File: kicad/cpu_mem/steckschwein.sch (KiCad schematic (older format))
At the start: 29 parts, among them P1 CONN_02X04, P3 CONN_01X03, P4 CONN_02X02, SW1 SW_PUSH, U1 W65C02SP, U2 LM555N, U3 74HCT00, U4 74LS393, U6 28C256, U7 HM62256BLP-7, U8 HM62256BLP-7, X1 OSC

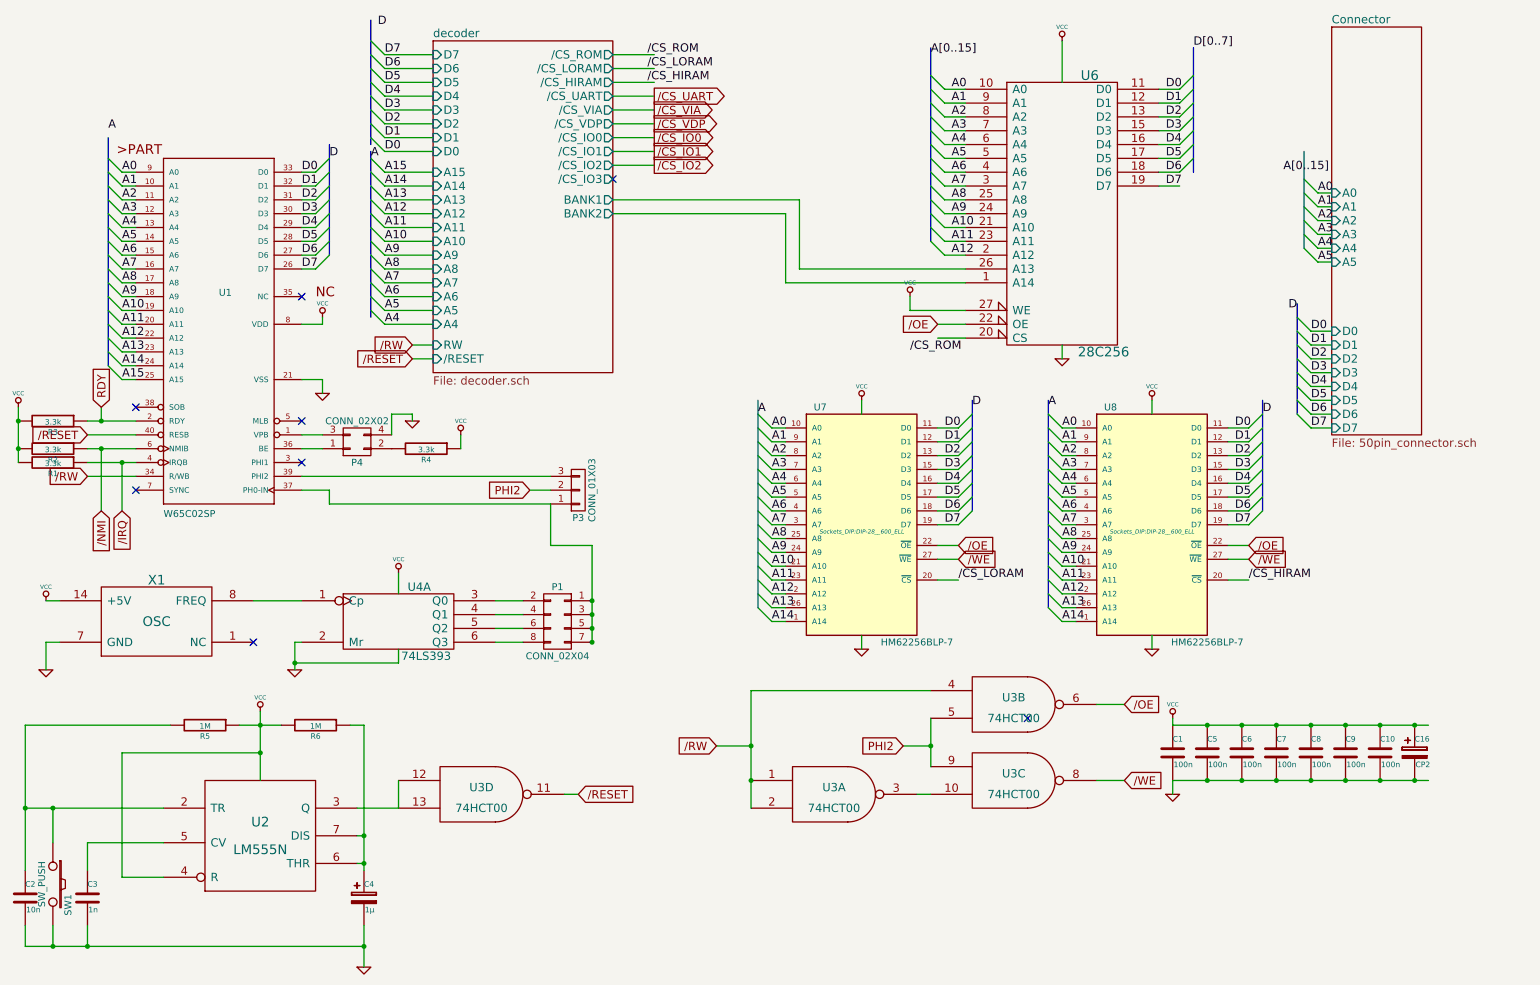
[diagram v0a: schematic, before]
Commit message: update
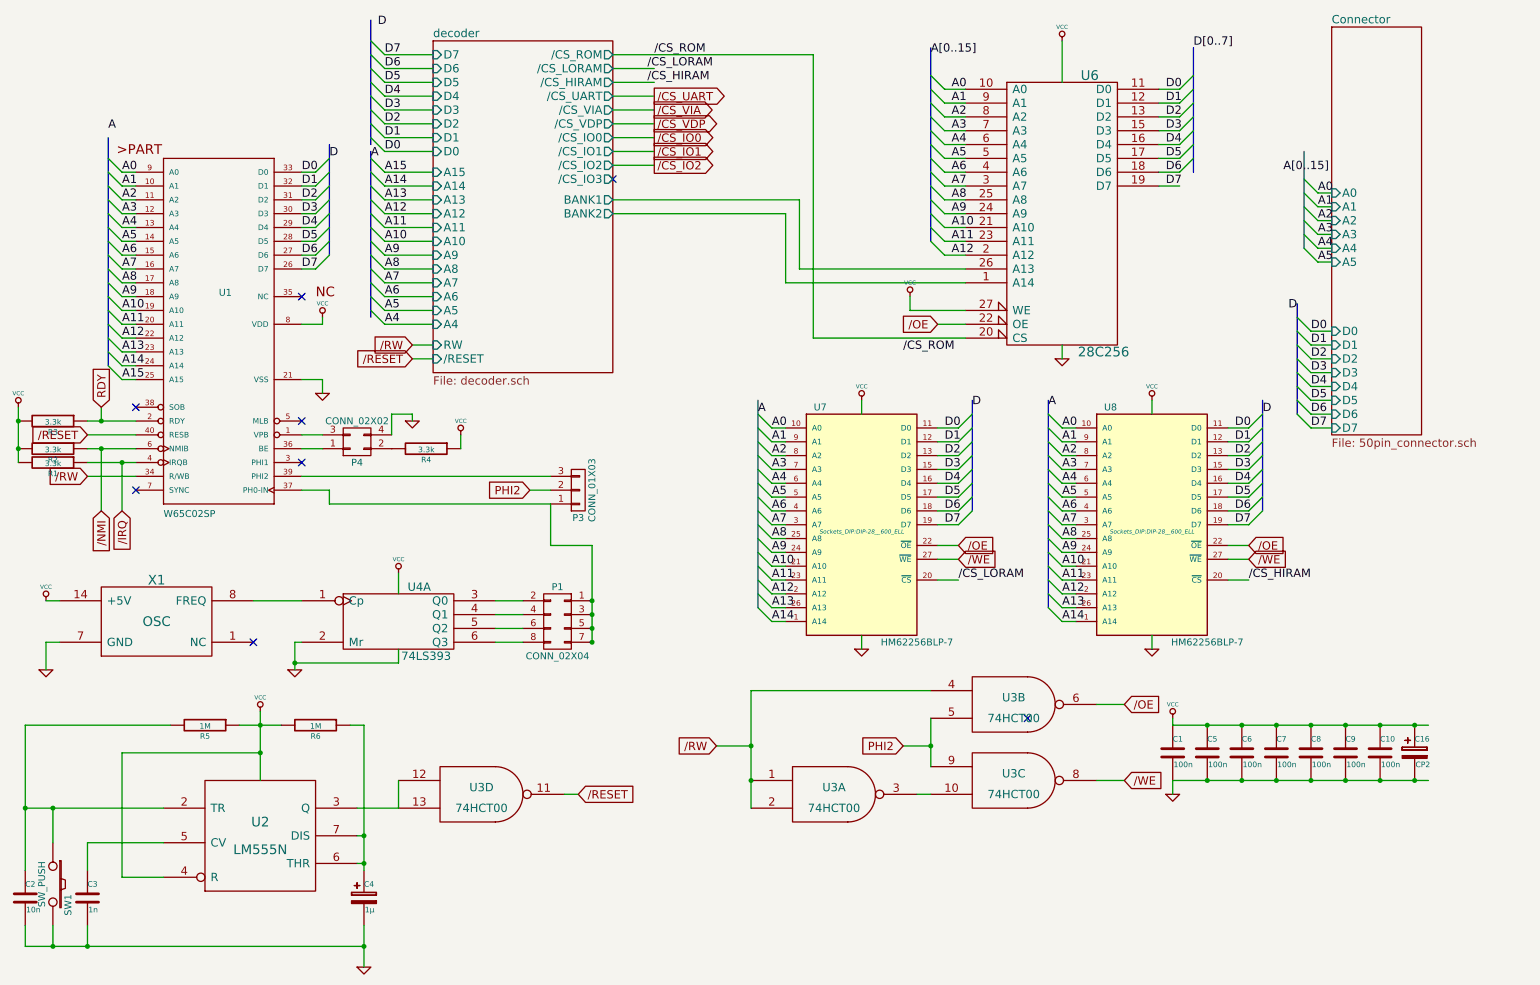
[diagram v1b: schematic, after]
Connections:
- net /CS_ROM: now also U6.20 (CS)
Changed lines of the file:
@@
 LIBS:ttl_ieee
 LIBS:steckschwein-cache
-EELAYER 24 0
+EELAYER 25 0
 EELAYER END
 $Descr A4 11693 8268
@@
 	1300 6750 1300 5850
 Wire Wire Line
-	2300 5850 1300 5850
+	1300 5850 2300 5850
 Connection ~ 2300 5850
 Wire Wire Line
@@
 Wire Wire Line
 	7400 2750 7200 2750
-Wire Wire Line
-	7400 2850 7200 2850
 Wire Bus Line
 	9050 750  9050 1650
@@
 Text Label 9450 4600 0    60   ~ 0
 /CS_HIRAM
-Text Label 7000 2950 0    60   ~ 0
-/CS_ROM
-Wire Wire Line
-	4850 800  5150 800
 Wire Wire Line
 	4850 900  5150 900
 Wire Wire Line
 	4850 1000 5150 1000
-Text Label 5100 800  0    60   ~ 0
-/CS_ROM
 Text Label 5100 900  0    60   ~ 0
 /CS_LORAM
@@
 	1    0    0    -1
 $EndComp
+Wire Wire Line
+	6300 2850 7400 2850
+Text Label 6950 2950 0    60   ~ 0
+/CS_ROM
+Wire Wire Line
+	4850 800  6300 800
+Text Label 5150 800  0    60   ~ 0
+/CS_ROM
+Wire Wire Line
+	6300 800  6300 2850
 $EndSCHEMATC
